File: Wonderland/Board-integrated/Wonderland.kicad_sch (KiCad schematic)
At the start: 292 parts, among them J1 Conn_01x03, J2 Conn_01x02, J3 Conn_01x03, U1 XC6206PxxxMR-Regulator_Linear, U2 W25Q32JVS, U3 RP2040, U4 USBLC6-2SC6, Y1 12MHz Crystal 3225

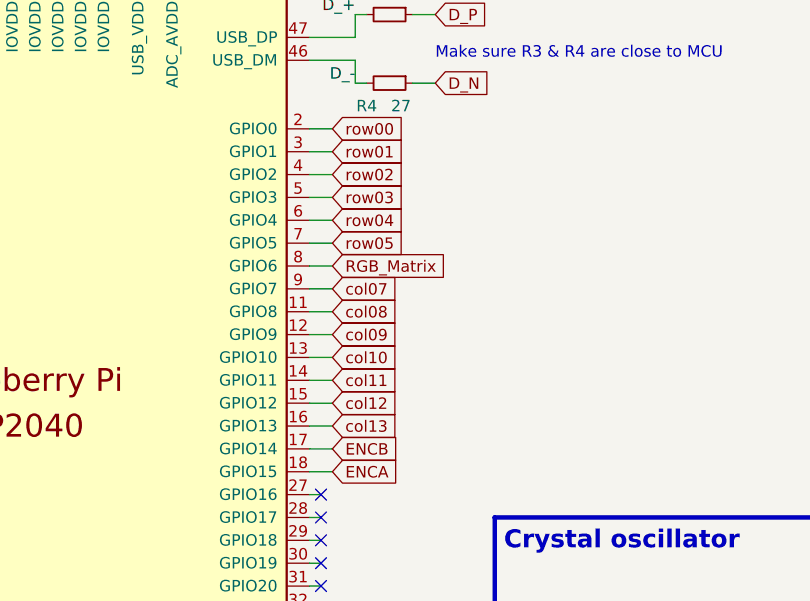
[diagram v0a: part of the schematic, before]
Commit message: edit pcb
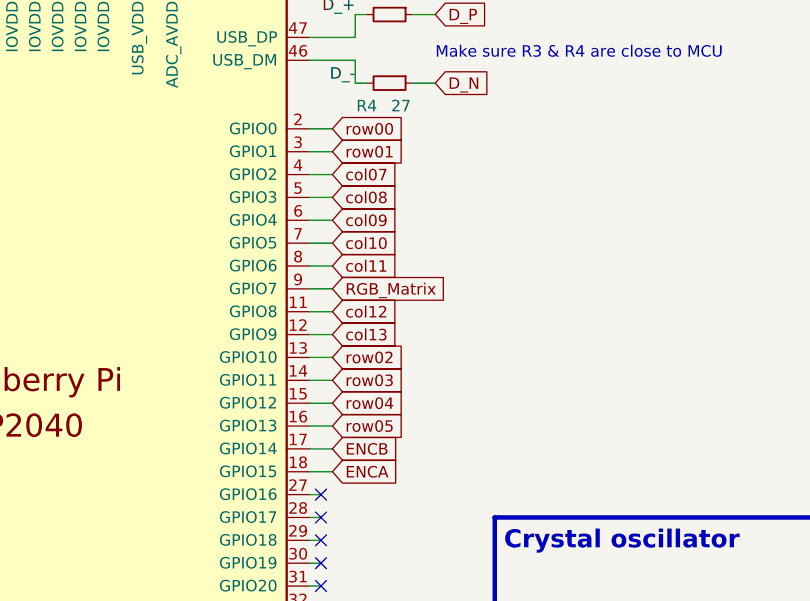
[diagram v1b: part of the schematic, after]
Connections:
- net RGB_Matrix: now also U3.9 (GPIO7); no longer U3.8 (GPIO6)
- net col07: now also U3.4 (GPIO2); no longer U3.9 (GPIO7)
- net col08: now also U3.5 (GPIO3); no longer U3.11 (GPIO8)
- net col09: now also U3.6 (GPIO4); no longer U3.12 (GPIO9)
- net col10: now also U3.7 (GPIO5); no longer U3.13 (GPIO10)
- net col11: now also U3.8 (GPIO6); no longer U3.14 (GPIO11)
- net col12: now also U3.11 (GPIO8); no longer U3.15 (GPIO12)
- net col13: now also U3.12 (GPIO9); no longer U3.16 (GPIO13)
- net row02: now also U3.13 (GPIO10); no longer U3.4 (GPIO2)
- net row03: now also U3.14 (GPIO11); no longer U3.5 (GPIO3)
- net row04: now also U3.15 (GPIO12); no longer U3.6 (GPIO4)
- net row05: now also U3.16 (GPIO13); no longer U3.7 (GPIO5)
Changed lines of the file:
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@@
     (stroke (width 0) (type default))
   )
-  (wire (pts (xy 105.41 332.74) (xy 102.87 332.74))
+  (wire (pts (xy 105.41 320.04) (xy 102.87 320.04))
     (stroke (width 0) (type default))
   )
@@
     (stroke (width 0) (type solid))
   )
-  (wire (pts (xy 105.41 325.12) (xy 102.87 325.12))
+  (wire (pts (xy 105.41 327.66) (xy 102.87 327.66))
     (stroke (width 0) (type default))
   )
@@
     (stroke (width 0) (type default))
   )
-  (wire (pts (xy 105.41 322.58) (xy 102.87 322.58))
+  (wire (pts (xy 105.41 342.9) (xy 102.87 342.9))
     (stroke (width 0) (type default))
   )
@@
     (stroke (width 0) (type default))
   )
-  (wire (pts (xy 105.41 317.5) (xy 102.87 317.5))
+  (wire (pts (xy 105.41 337.82) (xy 102.87 337.82))
     (stroke (width 0) (type default))
   )
@@
     (stroke (width 0) (type default))
   )
-  (wire (pts (xy 105.41 340.36) (xy 102.87 340.36))
+  (wire (pts (xy 105.41 330.2) (xy 102.87 330.2))
     (stroke (width 0) (type default))
   )
@@
     (stroke (width 0) (type default))
   )
-  (wire (pts (xy 105.41 327.66) (xy 102.87 327.66))
+  (wire (pts (xy 105.41 314.96) (xy 102.87 314.96))
     (stroke (width 0) (type default))
   )
@@
     (stroke (width 0) (type default))
   )
-  (wire (pts (xy 105.41 337.82) (xy 102.87 337.82))
+  (wire (pts (xy 105.41 325.12) (xy 102.87 325.12))
     (stroke (width 0) (type default))
   )
@@
     (stroke (width 0) (type default))
   )
-  (wire (pts (xy 105.41 335.28) (xy 102.87 335.28))
+  (wire (pts (xy 105.41 322.58) (xy 102.87 322.58))
     (stroke (width 0) (type default))
   )
@@
     (stroke (width 0) (type default))
   )
-  (wire (pts (xy 105.41 342.9) (xy 102.87 342.9))
+  (wire (pts (xy 105.41 332.74) (xy 102.87 332.74))
     (stroke (width 0) (type default))
   )
@@
     (stroke (width 0) (type default))
   )
-  (wire (pts (xy 105.41 330.2) (xy 102.87 330.2))
+  (wire (pts (xy 105.41 317.5) (xy 102.87 317.5))
     (stroke (width 0) (type default))
   )
@@
     (stroke (width 0) (type default))
   )
-  (wire (pts (xy 105.41 314.96) (xy 102.87 314.96))
+  (wire (pts (xy 105.41 335.28) (xy 102.87 335.28))
     (stroke (width 0) (type default))
   )
@@
     (stroke (width 0) (type default))
   )
-  (wire (pts (xy 105.41 320.04) (xy 102.87 320.04))
+  (wire (pts (xy 105.41 340.36) (xy 102.87 340.36))
     (stroke (width 0) (type default))
   )
@@
     )
   )
-  (global_label "row03" (shape input) (at 105.41 317.5 0) (fields_autoplaced)
+  (global_label "row03" (shape input) (at 105.41 337.82 0) (fields_autoplaced)
     (effects (font (size 1.27 1.27)) (justify left))
-    (property "Intersheetrefs" "${INTERSHEET_REFS}" (at 114.0799 317.5 0)
+    (property "Intersheetrefs" "${INTERSHEET_REFS}" (at 114.0799 337.82 0)
       (effects (font (size 1.27 1.27)) (justify left) hide)
     )
@@
     )
   )
-  (global_label "row04" (shape input) (at 105.41 320.04 0) (fields_autoplaced)
+  (global_label "row04" (shape input) (at 105.41 340.36 0) (fields_autoplaced)
     (effects (font (size 1.27 1.27)) (justify left))
-    (property "Intersheetrefs" "${INTERSHEET_REFS}" (at 114.0799 320.04 0)
+    (property "Intersheetrefs" "${INTERSHEET_REFS}" (at 114.0799 340.36 0)
       (effects (font (size 1.27 1.27)) (justify left) hide)
     )
@@
     )
   )
-  (global_label "col08" (shape input) (at 105.41 330.2 0) (fields_autoplaced)
+  (global_label "col08" (shape input) (at 105.41 317.5 0) (fields_autoplaced)
     (effects (font (size 1.27 1.27)) (justify left))
-    (property "Intersheetrefs" "${INTERSHEET_REFS}" (at 113.717 330.2 0)
+    (property "Intersheetrefs" "${INTERSHEET_REFS}" (at 113.717 317.5 0)
       (effects (font (size 1.27 1.27)) (justify left) hide)
     )
@@
     )
   )
-  (global_label "row02" (shape input) (at 105.41 314.96 0) (fields_autoplaced)
+  (global_label "row02" (shape input) (at 105.41 335.28 0) (fields_autoplaced)
     (effects (font (size 1.27 1.27)) (justify left))
-    (property "Intersheetrefs" "${INTERSHEET_REFS}" (at 114.0799 314.96 0)
+    (property "Intersheetrefs" "${INTERSHEET_REFS}" (at 114.0799 335.28 0)
       (effects (font (size 1.27 1.27)) (justify left) hide)
     )
@@
     )
   )
-  (global_label "RGB_Matrix" (shape input) (at 105.41 325.12 0) (fields_autoplaced)
+  (global_label "RGB_Matrix" (shape input) (at 105.41 327.66 0) (fields_autoplaced)
     (effects (font (size 1.27 1.27)) (justify left))
-    (property "Intersheetrefs" "${INTERSHEET_REFS}" (at 118.918 325.12 0)
+    (property "Intersheetrefs" "${INTERSHEET_REFS}" (at 118.918 327.66 0)
       (effects (font (size 1.27 1.27)) (justify left) hide)
     )
   )
-  (global_label "col13" (shape input) (at 105.41 342.9 0) (fields_autoplaced)
+  (global_label "col13" (shape input) (at 105.41 332.74 0) (fields_autoplaced)
     (effects (font (size 1.27 1.27)) (justify left))
-    (property "Intersheetrefs" "${INTERSHEET_REFS}" (at 113.717 342.9 0)
+    (property "Intersheetrefs" "${INTERSHEET_REFS}" (at 113.717 332.74 0)
       (effects (font (size 1.27 1.27)) (justify left) hide)
     )
@@
     )
   )
-  (global_label "row05" (shape input) (at 105.41 322.58 0) (fields_autoplaced)
+  (global_label "row05" (shape input) (at 105.41 342.9 0) (fields_autoplaced)
     (effects (font (size 1.27 1.27)) (justify left))
-    (property "Intersheetrefs" "${INTERSHEET_REFS}" (at 114.0799 322.58 0)
+    (property "Intersheetrefs" "${INTERSHEET_REFS}" (at 114.0799 342.9 0)
       (effects (font (size 1.27 1.27)) (justify left) hide)
     )
@@
     )
   )
-  (global_label "col12" (shape input) (at 105.41 340.36 0) (fields_autoplaced)
+  (global_label "col12" (shape input) (at 105.41 330.2 0) (fields_autoplaced)
     (effects (font (size 1.27 1.27)) (justify left))
-    (property "Intersheetrefs" "${INTERSHEET_REFS}" (at 113.717 340.36 0)
+    (property "Intersheetrefs" "${INTERSHEET_REFS}" (at 113.717 330.2 0)
       (effects (font (size 1.27 1.27)) (justify left) hide)
     )
@@
     )
   )
-  (global_label "col07" (shape input) (at 105.41 327.66 0) (fields_autoplaced)
+  (global_label "col07" (shape input) (at 105.41 314.96 0) (fields_autoplaced)
     (effects (font (size 1.27 1.27)) (justify left))
-    (property "Intersheetrefs" "${INTERSHEET_REFS}" (at 113.717 327.66 0)
+    (property "Intersheetrefs" "${INTERSHEET_REFS}" (at 113.717 314.96 0)
       (effects (font (size 1.27 1.27)) (justify left) hide)
     )
@@
     )
   )
-  (global_label "col11" (shape input) (at 105.41 337.82 0) (fields_autoplaced)
+  (global_label "col11" (shape input) (at 105.41 325.12 0) (fields_autoplaced)
     (effects (font (size 1.27 1.27)) (justify left))
-    (property "Intersheetrefs" "${INTERSHEET_REFS}" (at 113.717 337.82 0)
+    (property "Intersheetrefs" "${INTERSHEET_REFS}" (at 113.717 325.12 0)
       (effects (font (size 1.27 1.27)) (justify left) hide)
     )
   )
-  (global_label "col09" (shape input) (at 105.41 332.74 0) (fields_autoplaced)
+  (global_label "col09" (shape input) (at 105.41 320.04 0) (fields_autoplaced)
     (effects (font (size 1.27 1.27)) (justify left))
-    (property "Intersheetrefs" "${INTERSHEET_REFS}" (at 113.717 332.74 0)
+    (property "Intersheetrefs" "${INTERSHEET_REFS}" (at 113.717 320.04 0)
       (effects (font (size 1.27 1.27)) (justify left) hide)
     )
@@
     )
   )
-  (global_label "col10" (shape input) (at 105.41 335.28 0) (fields_autoplaced)
+  (global_label "col10" (shape input) (at 105.41 322.58 0) (fields_autoplaced)
     (effects (font (size 1.27 1.27)) (justify left))
-    (property "Intersheetrefs" "${INTERSHEET_REFS}" (at 113.717 335.28 0)
+    (property "Intersheetrefs" "${INTERSHEET_REFS}" (at 113.717 322.58 0)
       (effects (font (size 1.27 1.27)) (justify left) hide)
     )

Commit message: generated PCB
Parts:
- added RGBI0, RGBI1, RGBI2: SK6812MINI-E, Keyboard:SK6812-MINI-E_back, symbol Keyboard:SK6812MINI-E
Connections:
- net +3V3: now also RGBI0.1 (VCC), RGBI1.1 (VCC), RGBI2.1 (VCC)
- net GND: now also RGBI0.3 (GND), RGBI1.3 (GND), RGBI2.3 (GND)
- net RGB_Out: now also RGBI2.2 (DOUT); no longer RGBF0.2 (DOUT)
- new net IN_I0: RGBF0.2 (DOUT), RGBI0.4 (DIN)
- new net IN_I1: RGBI0.2 (DOUT), RGBI1.4 (DIN)
- new net IN_I2: RGBI1.2 (DOUT), RGBI2.4 (DIN)
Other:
- moved on the sheet: J3

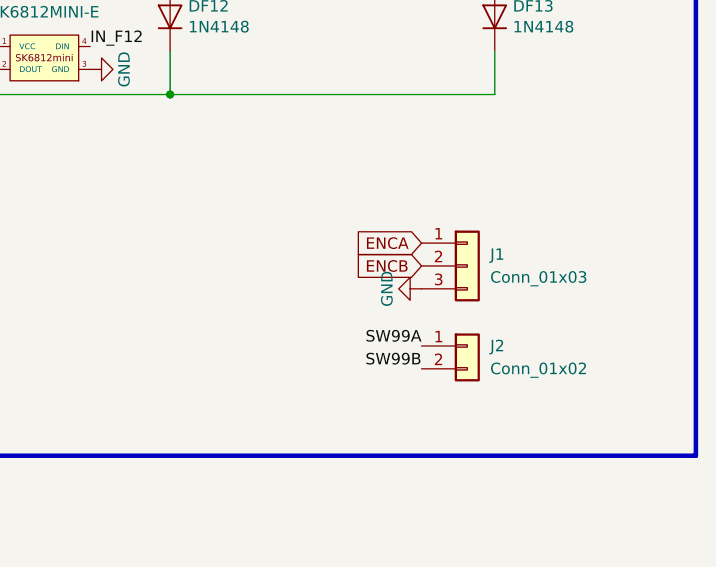
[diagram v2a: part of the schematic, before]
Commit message: update wonderland
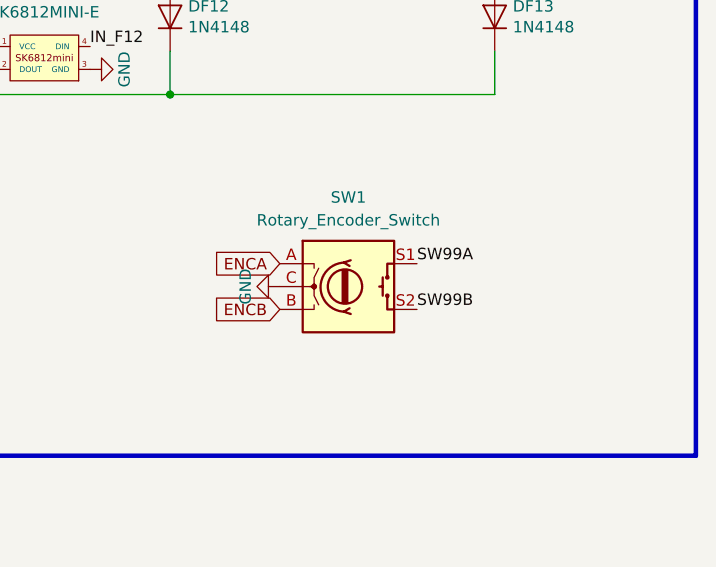
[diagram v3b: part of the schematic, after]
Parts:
- removed J1: Conn_01x03, Keyboard:PinHeader_1x03_P2.54mm_Vertical, symbol Keyboard:Conn_01x03
- removed J2: Conn_01x02, Keyboard:PinHeader_1x02_P2.54mm_Vertical, symbol Keyboard:Conn_01x02
- added SW1: Rotary_Encoder_Switch, Keyboard:RotaryEncoder_EC11-Switch_Horizontal_H15mm, symbol Keyboard:Rotary_Encoder_Switch
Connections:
- net ENCA: now also SW1.A
- net ENCB: now also SW1.B
- net GND: now also SW1.C
- net SW99B: now also SW1.S2
- net col13: now also SW1.S1
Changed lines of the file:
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@@
     (effects (font (size 1.27 1.27)) (justify right bottom))
   )
-  (label "SW99A" (at 530.86 200.914 180) (fields_autoplaced)
-    (effects (font (size 1.27 1.27)) (justify right bottom))
+  (label "SW99A" (at 530.352 191.77 0) (fields_autoplaced)
+    (effects (font (size 1.27 1.27)) (justify left bottom))
   )
   (label "IN_A11" (at 458.47 49.53 0) (fields_autoplaced)
@@
     (effects (font (size 1.27 1.27)) (justify left bottom))
   )
-  (label "SW99B" (at 530.86 203.454 180) (fields_autoplaced)
-    (effects (font (size 1.27 1.27)) (justify right bottom))
+  (label "SW99B" (at 530.352 196.85 0) (fields_autoplaced)
+    (effects (font (size 1.27 1.27)) (justify left bottom))
   )
   (label "OUT_E4" (at 193.04 146.05 180) (fields_autoplaced)
@@
     )
   )
-  (global_label "ENCB" (shape input) (at 530.86 192.024 180) (fields_autoplaced)
+  (global_label "ENCB" (shape input) (at 515.112 196.85 180) (fields_autoplaced)
     (effects (font (size 1.27 1.27)) (justify right))
-    (property "Intersheetrefs" "${INTERSHEET_REFS}" (at 447.548 130.556 0)
+    (property "Intersheetrefs" "${INTERSHEET_REFS}" (at 431.8 135.382 0)
       (effects (font (size 1.27 1.27)) hide)
     )
@@
     )
   )
-  (global_label "ENCA" (shape input) (at 530.86 189.484 180) (fields_autoplaced)
+  (global_label "ENCA" (shape input) (at 515.112 191.77 180) (fields_autoplaced)
     (effects (font (size 1.27 1.27)) (justify right))
-    (property "Intersheetrefs" "${INTERSHEET_REFS}" (at 447.548 133.096 0)
+    (property "Intersheetrefs" "${INTERSHEET_REFS}" (at 431.8 135.382 0)
       (effects (font (size 1.27 1.27)) hide)
     )
@@
     )
   )
-  (symbol (lib_id "power:GND") (at 530.86 194.564 270) (unit 1)
+  (symbol (lib_id "power:GND") (at 515.112 194.31 270) (unit 1)
     (in_bom yes) (on_board yes) (dnp no)
-    (property "Reference" "#PWR0243" (at 524.51 194.564 0)
+    (property "Reference" "#PWR0243" (at 508.762 194.31 0)
       (effects (font (size 1.27 1.27)) hide)
     )
-    (property "Value" "GND" (at 527.05 194.564 0)
+    (property "Value" "GND" (at 511.302 194.31 0)
       (effects (font (size 1.27 1.27)))
     )
-    (property "Footprint" "" (at 530.86 194.564 0)
+    (property "Footprint" "" (at 515.112 194.31 0)
       (effects (font (size 1.27 1.27)) hide)
     )
-    (property "Datasheet" "" (at 530.86 194.564 0)
+    (property "Datasheet" "" (at 515.112 194.31 0)
       (effects (font (size 1.27 1.27)) hide)
     )
@@
     )
   )
+  (symbol (lib_id "Keyboard:Rotary_Encoder_Switch") (at 522.732 194.31 0) (unit 1)
+    (in_bom yes) (on_board yes) (dnp no) (fields_autoplaced)
+    (property "Reference" "SW1" (at 522.732 184.404 0)
+      (effects (font (size 1.27 1.27)))
+    )
+    (property "Value" "Rotary_Encoder_Switch" (at 522.732 186.944 0)
+      (effects (font (size 1.27 1.27)))
+    )
+    (property "Footprint" "Keyboard:RotaryEncoder_EC11-Switch_Horizontal_H15mm" (at 531.622 202.946 0)
+      (effects (font (size 1.27 1.27)) hide)
+    )
+    (property "Datasheet" "" (at 522.732 187.706 0)
+      (effects (font (size 1.27 1.27)) hide)
+    )
+    (pin "S2")
+    (pin "B")
+    (pin "S1")
+    (pin "C")
+    (pin "A")
+    (instances
+      (project "Wonderland"
+        (path "/ba62e47e-9e07-4e97-ab08-24b670d50f97"
+          (reference "SW1") (unit 1)
+        )
+      )
+    )
+  )
   (symbol (lib_name "+3V3_61") (lib_id "power:+3V3") (at 193.04 72.39 90) (unit 1)
     (in_bom yes) (on_board yes) (dnp no)
@@
     )
   )
-  (symbol (lib_id "Keyboard:Conn_01x02") (at 535.94 200.914 0) (unit 1)
-    (in_bom yes) (on_board yes) (dnp no) (fields_autoplaced)
-    (property "Reference" "J2" (at 538.48 200.914 0)
-      (effects (font (size 1.27 1.27)) (justify left))
-    )
-    (property "Value" "Conn_01x02" (at 538.48 203.454 0)
-      (effects (font (size 1.27 1.27)) (justify left))
-    )
-    (property "Footprint" "Keyboard:PinHeader_1x02_P2.54mm_Vertical" (at 535.94 200.914 0)
-      (effects (font (size 1.27 1.27)) hide)
-    )
-    (property "Datasheet" "~" (at 535.94 200.914 0)
-      (effects (font (size 1.27 1.27)) hide)
-    )
-    (pin "1")
-    (pin "2")
-    (instances
-      (project "Wonderland"
-        (path "/ba62e47e-9e07-4e97-ab08-24b670d50f97"
-          (reference "J2") (unit 1)
-        )
-      )
-    )
-  )
   (symbol (lib_id "Keyboard:SK6812MINI-E") (at 271.78 50.8 0) (unit 1)
     (in_bom yes) (on_board yes) (dnp no) (fields_autoplaced)
@@
         )
       )
-    )
-  )
-  (symbol (lib_id "Keyboard:Conn_01x03") (at 535.94 192.024 0) (unit 1)
-    (in_bom yes) (on_board yes) (dnp no) (fields_autoplaced)
-    (property "Reference" "J1" (at 538.48 190.754 0)
-      (effects (font (size 1.27 1.27)) (justify left))
-    )
-    (property "Value" "Conn_01x03" (at 538.48 193.294 0)
-      (effects (font (size 1.27 1.27)) (justify left))
-    )
-    (property "Footprint" "Keyboard:PinHeader_1x03_P2.54mm_Vertical" (at 539.75 199.644 0)
-      (effects (font (size 1.27 1.27)) hide)
-    )
-    (property "Datasheet" "" (at 535.94 192.024 0)
-      (effects (font (size 1.27 1.27)) hide)
-    )
-    (pin "1")
-    (pin "2")
-    (pin "3")
-    (instances
-      (project "Wonderland"
-        (path "/ba62e47e-9e07-4e97-ab08-24b670d50f97"
-          (reference "J1") (unit 1)
-        )
-      )
